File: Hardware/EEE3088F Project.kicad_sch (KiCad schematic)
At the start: 41 parts, among them U1 OP1177ARM, U2 OP1177ARM, U3 OP1177ARM, U4 OP1177ARM, U5 OP1177ARM, U6 OP1177ARM

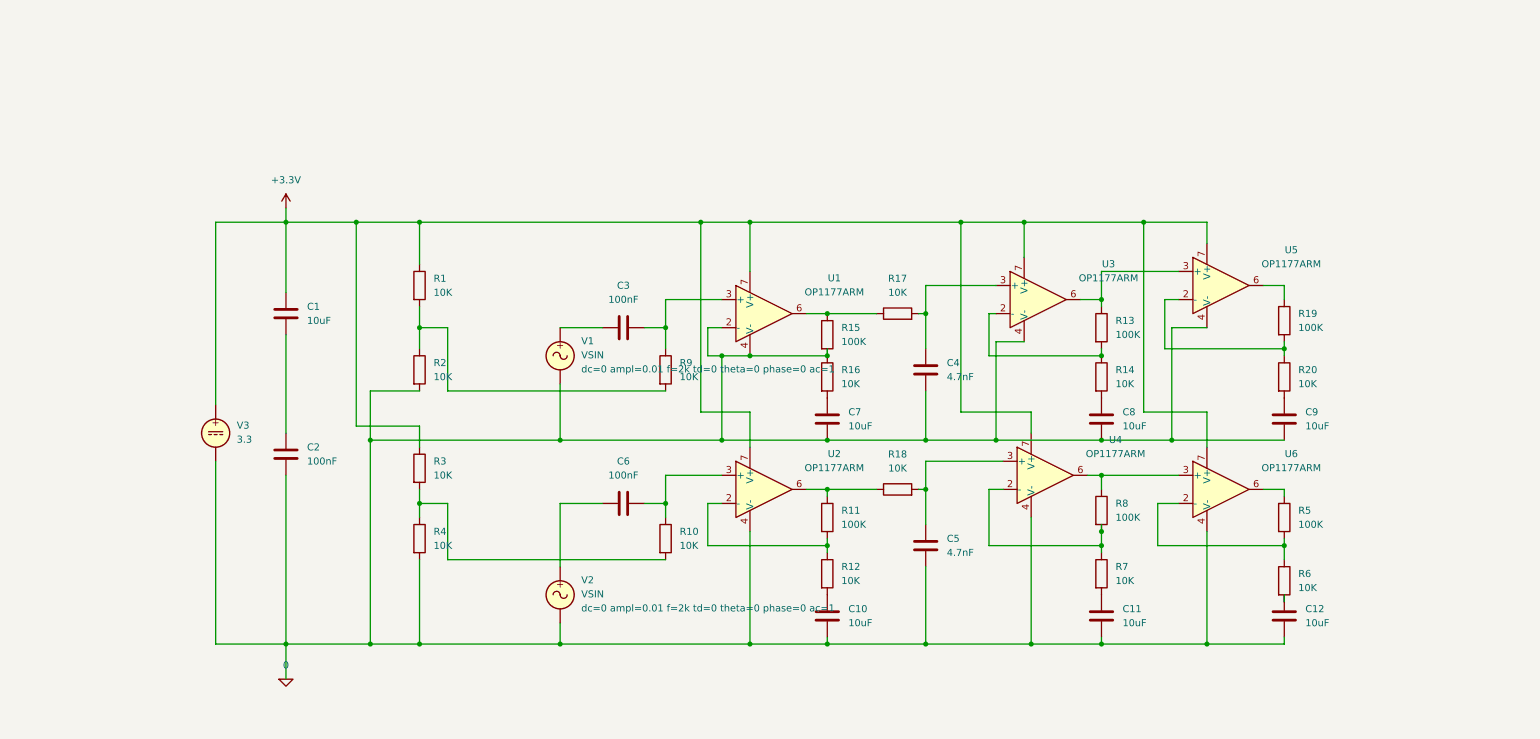
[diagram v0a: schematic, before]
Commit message: Upload updated files
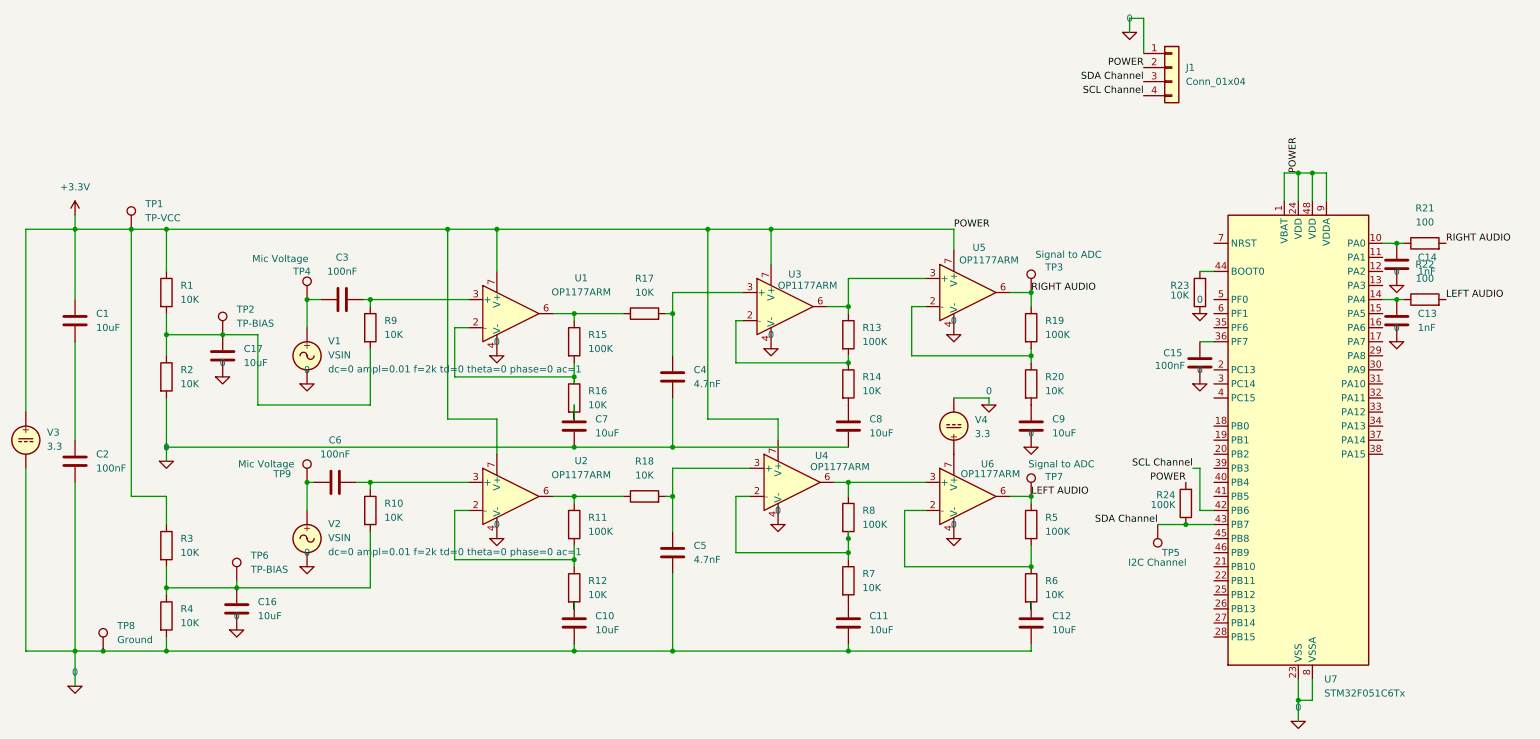
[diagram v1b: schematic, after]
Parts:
- added C13, C14: 1nF, symbol Device:C
- added C15: 100nF, symbol Device:C
- added C16, C17: 10uF, symbol Device:C
- added J1: Conn_01x04, symbol Connector_Generic:Conn_01x04
- added R21, R22: 100, Resistor_SMD:R_0201_0603Metric, symbol Device:R
- added R23: 10K, Resistor_SMD:R_0201_0603Metric, symbol Device:R
- added R24: 100K, Resistor_SMD:R_0201_0603Metric, symbol Device:R
- added TP1: TP-VCC, symbol Connector:TestPoint
- added TP2, TP6: TP-BIAS, symbol Connector:TestPoint
- added TP3, TP7: Signal to ADC, symbol Connector:TestPoint
- added TP4, TP9: Mic Voltage, symbol Connector:TestPoint
- added TP5: I2C Channel, symbol Connector:TestPoint
- added TP8: Ground, symbol Connector:TestPoint
- added U7: STM32F051C6Tx, Package_QFP:LQFP-48_7x7mm_P0.5mm, symbol MCU_ST_STM32F0:STM32F051C6Tx
- added V4: 3.3, symbol Simulation_SPICE:VDC
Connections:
- net +3.3V: now also J1.2 (Pin_2), R24.2, TP1.1, U7.1 (VBAT), U7.24 (VDD), U7.48 (VDD), U7.9 (VDDA); no longer U6.7 (V+)
- net 0: now also C13.2, C14.2, C15.2, C16.1, C17.1, J1.1 (Pin_1), R23.1, TP8.1, U7.23 (VSS), U7.47 (VSS), U7.8 (VSSA), V4.2; no longer R15.2, R16.1, U1.2 (-)
- net at R1.2, R2.1, R9.2: now also C17.2, TP2.1
- net LEFT AUDIO: now reaches R5.1, U6.6
- net LEFT AUDIO: now also R22.2, TP7.1
- net at R10.2, R3.2, R4.1: now also C16.2, TP6.1
- net at C6.1, V2.1: now also TP9.1
- net at C3.1, V1.1: now also TP4.1
- net RIGHT AUDIO: now reaches R19.1, U5.6
- net RIGHT AUDIO: now also R21.2, TP3.1
- new net: R15.2, R16.1, U1.2 (-)
- new net: C13.1, R22.1, U7.14 (PA4)
- new net: U6.7 (V+), V4.1
- new net: C15.1, U7.36 (PF7)
- new net: R23.2, U7.44 (BOOT0)
- new net: C14.1, R21.1, U7.10 (PA0)
- new net SCL Channel: J1.4 (Pin_4), U7.42 (PB6)
- new net SDA Channel: J1.3 (Pin_3), R24.1, TP5.1, U7.43 (PB7)
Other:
- moved on the sheet: C1, C10, C11, C12, C2, C3, C4, C5, C6, C7, C8, C9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
